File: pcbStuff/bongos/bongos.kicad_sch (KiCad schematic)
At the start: 11 parts, among them U1 74LS04, U2 74LS04, U3 74LS08, U4 74LS74, U5 74LS74, U6 74LS08, U7 74LS00

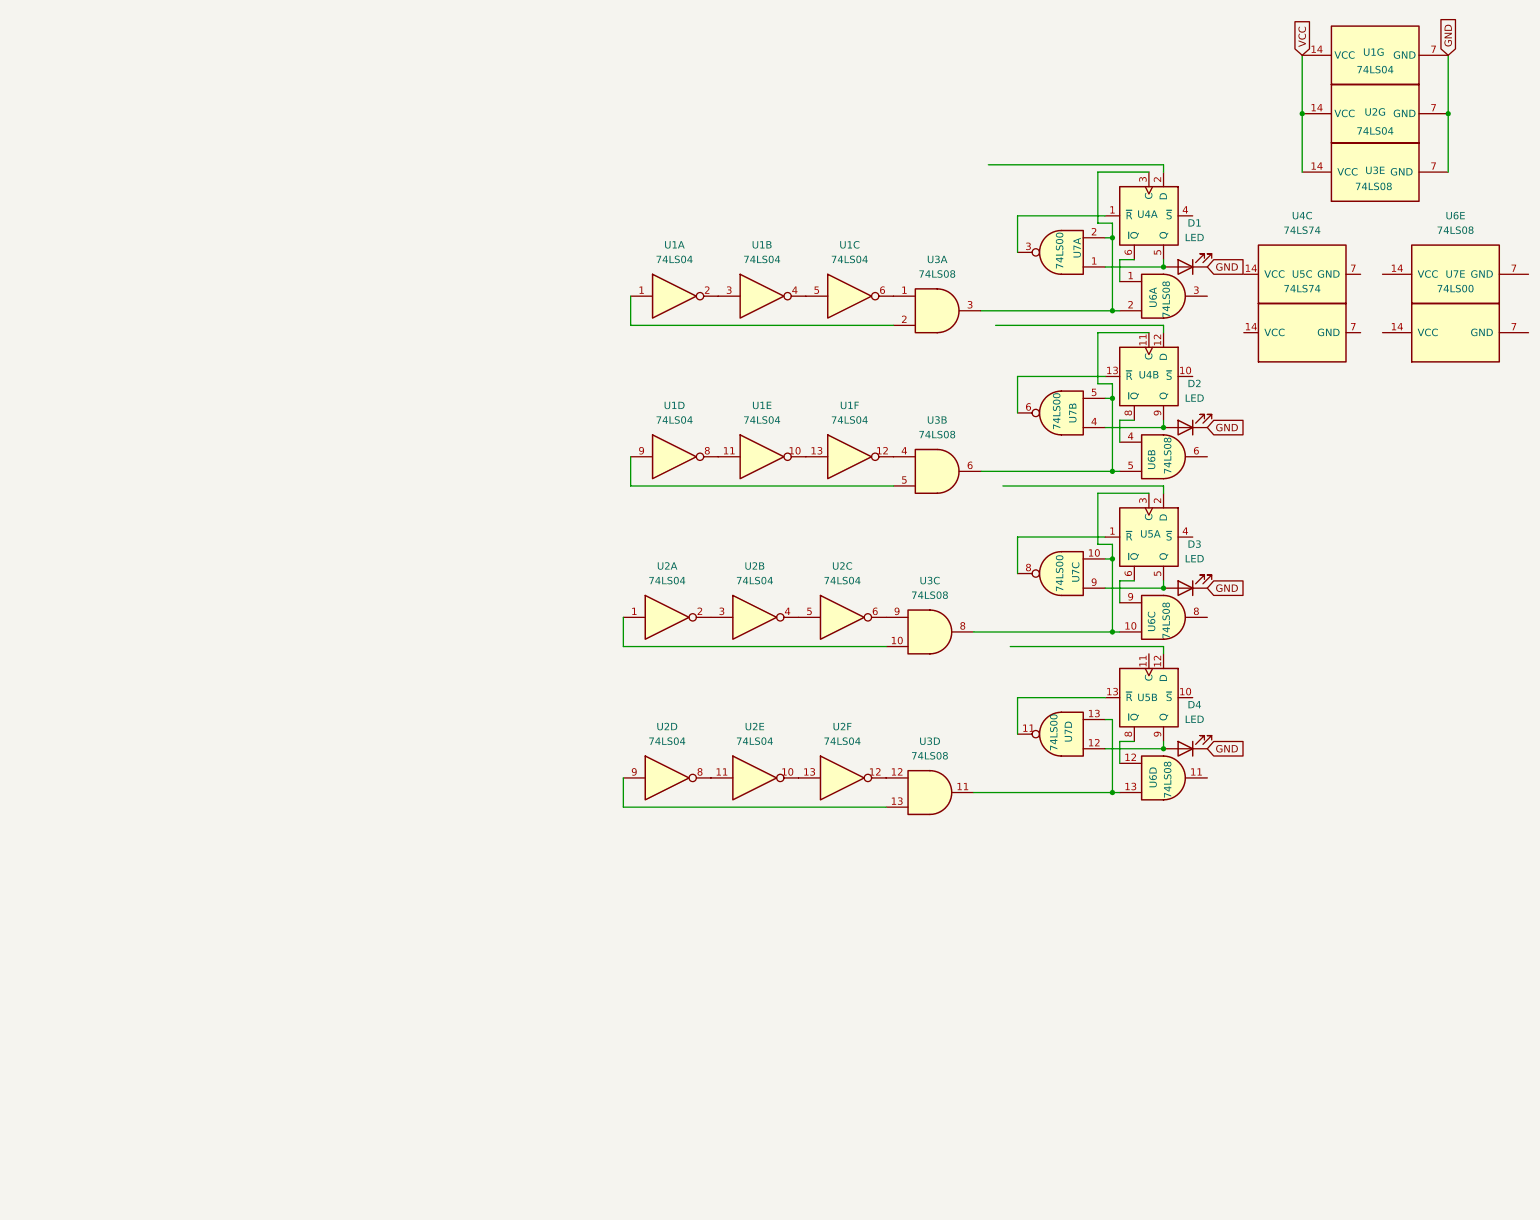
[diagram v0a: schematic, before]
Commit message: beauty is in the eye of the beholder
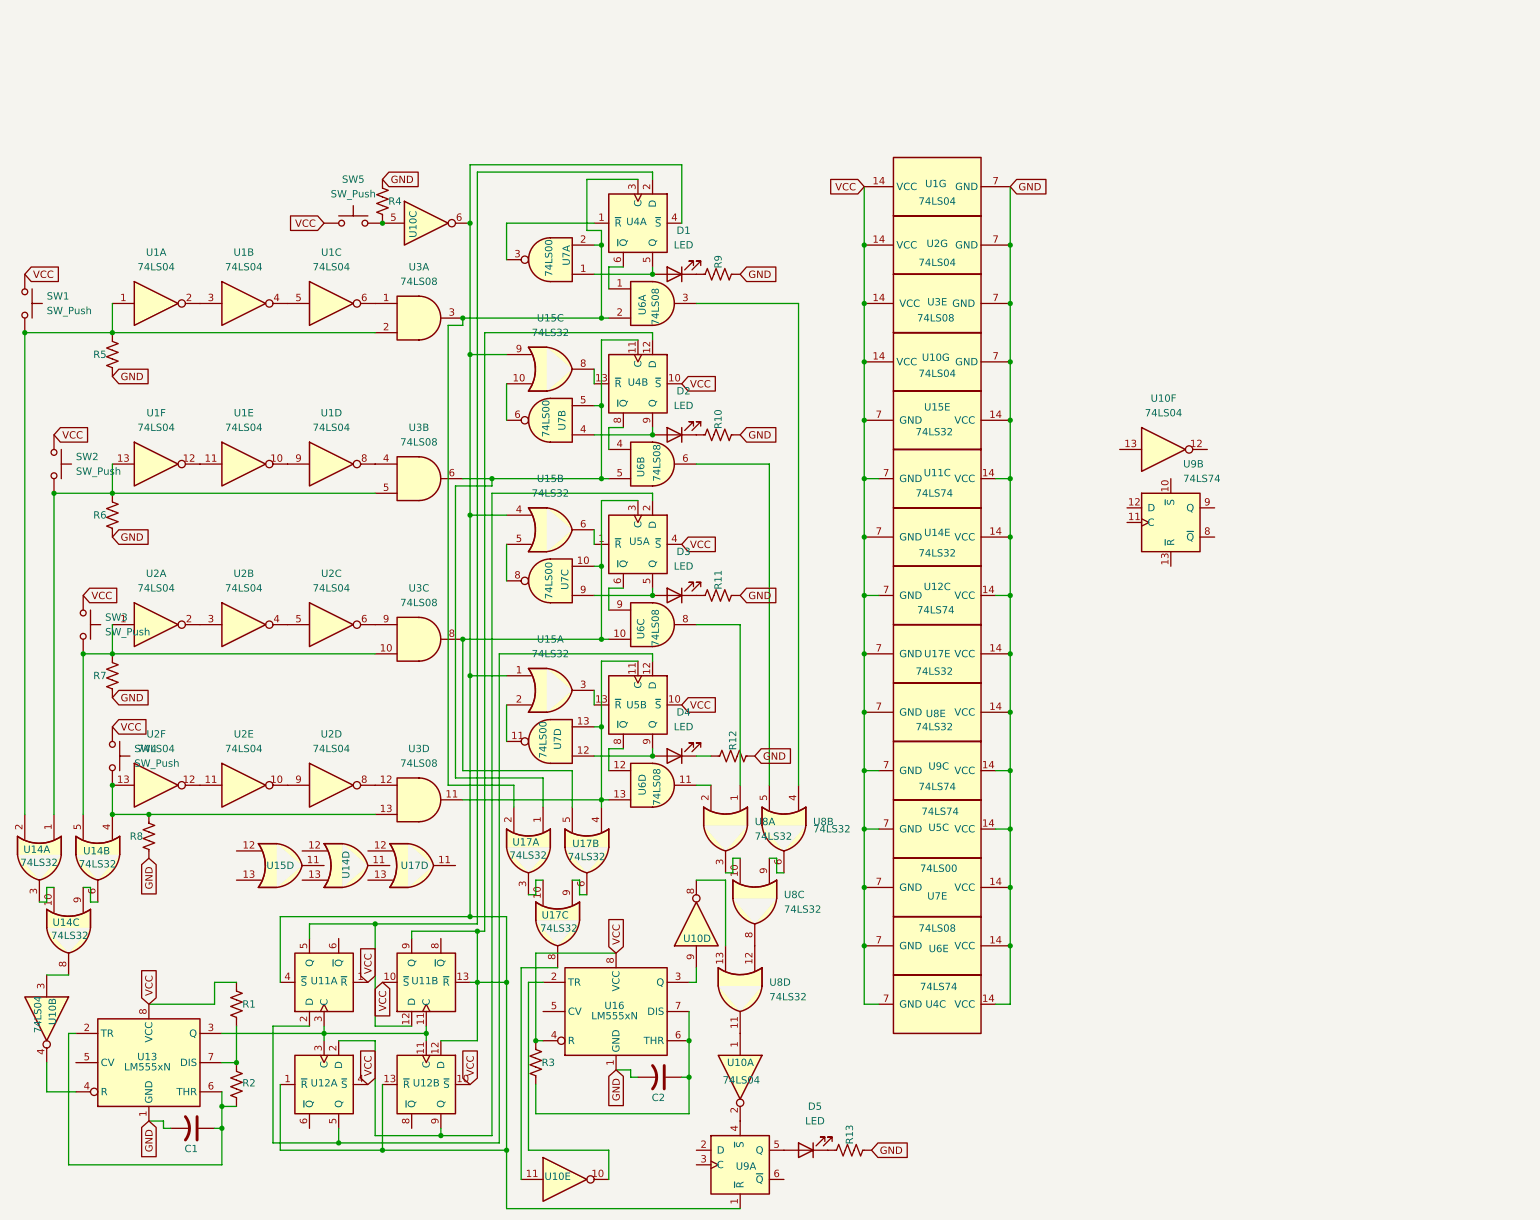
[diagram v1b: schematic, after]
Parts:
- added C1, C2: C_US, Capacitor_THT:CP_Radial_D5.0mm_P2.50mm, symbol Device:C_US
- added D5: LED, LED_THT:LED_D5.0mm, symbol Device:LED
- added R1, R10, R11, R12, R13, R2, R3, R4, R5, R6, R7, R8, R9: R_US, Resistor_THT:R_Axial_DIN0207_L6.3mm_D2.5mm_P7.62mm_Horizontal, symbol Device:R_US
- added SW1, SW2, SW3, SW4: SW_Push, Button_Switch_THT:SW_PUSH-12mm, symbol Switch:SW_Push
- added SW5: SW_Push, Button_Switch_THT:SW_PUSH_6mm, symbol Switch:SW_Push
- added U10: 74LS04, Package_DIP:DIP-14_W7.62mm, symbol 74xx:74LS04
- added U11, U12, U9: 74LS74, Package_DIP:DIP-14_W7.62mm, symbol 74xx:74LS74
- added U13, U16: LM555xN, Package_DIP:DIP-8_W7.62mm, symbol Timer:LM555xN
- added U14, U15, U17, U8: 74LS32, Package_DIP:DIP-14_W7.62mm, symbol 74xx:74LS32
- D1, D2, D3, D4: footprint (none) -> LED_THT:LED_D5.0mm
- U1, U2, U3, U4, U5, U6, U7: footprint (none) -> Package_DIP:DIP-14_W7.62mm
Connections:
- net GND: now also U4.14 (VCC), U5.14 (VCC), U6.14 (VCC), U7.14 (VCC), C1.2, C2.2, R10.2, R11.2, R12.2, R13.2, R4.1, R5.1, R6.1, R7.1, R8.1, R9.2, U10.7 (GND), U11.14 (VCC), U12.14 (VCC), U13.1 (GND), U14.14 (VCC), U15.14 (VCC), U16.1 (GND), U17.14 (VCC), U8.14 (VCC), U9.14 (VCC); no longer D1.1 (K), D2.1 (K), D3.1 (K), D4.1 (K)
- net VCC: now also U4.10 (~{S}), U4.7 (GND), U5.10 (~{S}), U5.4 (~{S}), U5.7 (GND), U6.7 (GND), U7.7 (GND), R1.1, R3.1, SW1.1, SW2.1, SW3.1, SW4.1, SW5.1, U10.14 (VCC), U11.1 (~{R}), U11.10 (~{S}), U11.7 (GND), U12.10 (~{S}), U12.4 (~{S}), U12.7 (GND), U13.8 (VCC), U14.7 (GND), U15.7 (GND), U16.4 (R), U16.8 (VCC), U17.7 (GND), U8.7 (GND), U9.7 (GND)
- net at U2.1, U3.10: now also R7.2, SW3.2, U14.5
- net at U3.6, U4.11 (C), U6.5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: now also U17.1
- net at U7.6: now also U15.10; no longer U4.13 (~{R})
- net at U3.11, U6.13, U7.13: now also U5.11 (C), U17.4
- net at U3.12: now also U2.8; no longer U2.12
- net at U3.13: now also U2.13, R8.2, SW4.2, U14.4; no longer U2.9
- net at U2.11: now also U2.12; no longer U2.8
- net at U7.11: now also U15.2; no longer U5.13 (~{R})
- net at U6.6: now also U8.5
- net at U1.1, U3.2: now also R5.2, SW1.2, U14.2
- net at U2.10: now also U2.9; no longer U2.13
- net at U1.12: now also U1.11; no longer U3.4
- net at U1.13: now also U3.5, R6.2, SW2.2, U14.1; no longer U1.10
- net at U3.3, U4.3 (C), U6.2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: now also U17.2
- net at U6.3: now also U8.4
- net at U5.1 (~{R}): now also U15.6; no longer U7.8
- net at U5.2 (D): now also U12.2 (D), U12.9 (Q)
- net at U3.8, U5.3 (C), U6.10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: now also U17.5
- net at U4.12 (D): now also U4.4 (~{S}), U10.6, U11.13 (~{R}), U11.4 (~{S}), U11.9 (Q), U12.1 (~{R}), U12.12 (D), U12.13 (~{R}), U15.1, U15.4, U15.9, U9.1 (~{R})
- net at U5.12 (D): now also U11.2 (D), U12.5 (Q)
- net at U1.8: now also U3.4; no longer U1.11
- net at U6.11: now also U8.2
- net at U4.2 (D): now also U11.12 (D), U11.5 (Q)
- net at U1.9: now also U1.10; no longer U3.5
- net at U6.8: now also U8.1
- new net: D1.1 (K), R9.1
- new net: R4.2, SW5.2, U10.5
- new net: U11.11 (C), U11.3 (C), U12.11 (C), U12.3 (C), U13.3 (Q)
- new net: U8.10, U8.3
- new net: U8.12, U8.8
- new net: U8.6, U8.9
- new net: U10.2, U9.4 (~{S})
- new net: D5.2 (A), U9.5 (Q)
- new net: R1.2, R2.1, U13.7 (DIS)
- new net: U10.8, U8.13
- new net: U10.9, U16.3 (Q)
- new net: D4.1 (K), R12.1
- new net: C2.1, R3.2, U16.6 (THR), U16.7 (DIS)
- new net: D5.1 (K), R13.1
- new net: U10.3, U14.8
- new net: U10.4, U13.4 (R)
- new net: C1.1, R2.2, U13.2 (TR), U13.6 (THR)
- new net: U10.1, U8.11
- new net: U15.3, U5.13 (~{R})
- new net: U10.10, U16.2 (TR)
- new net: U17.10, U17.3
- new net: U10.11, U17.8
- new net: U17.6, U17.9
- new net: U15.8, U4.13 (~{R})
- new net: U14.10, U14.3
- new net: U14.6, U14.9
- new net: D3.1 (K), R11.1
- new net: U15.5, U7.8
- new net: D2.1 (K), R10.1
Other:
- moved on the sheet: D1, D2, D3, D4, U1A, U1B, U1C, U1D, U1E, U1F, U1G, U2A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
